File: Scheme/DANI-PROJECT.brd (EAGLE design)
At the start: 59.7 x 81 mm, 29 parts, among them T1 2N2222, T2 2N2222

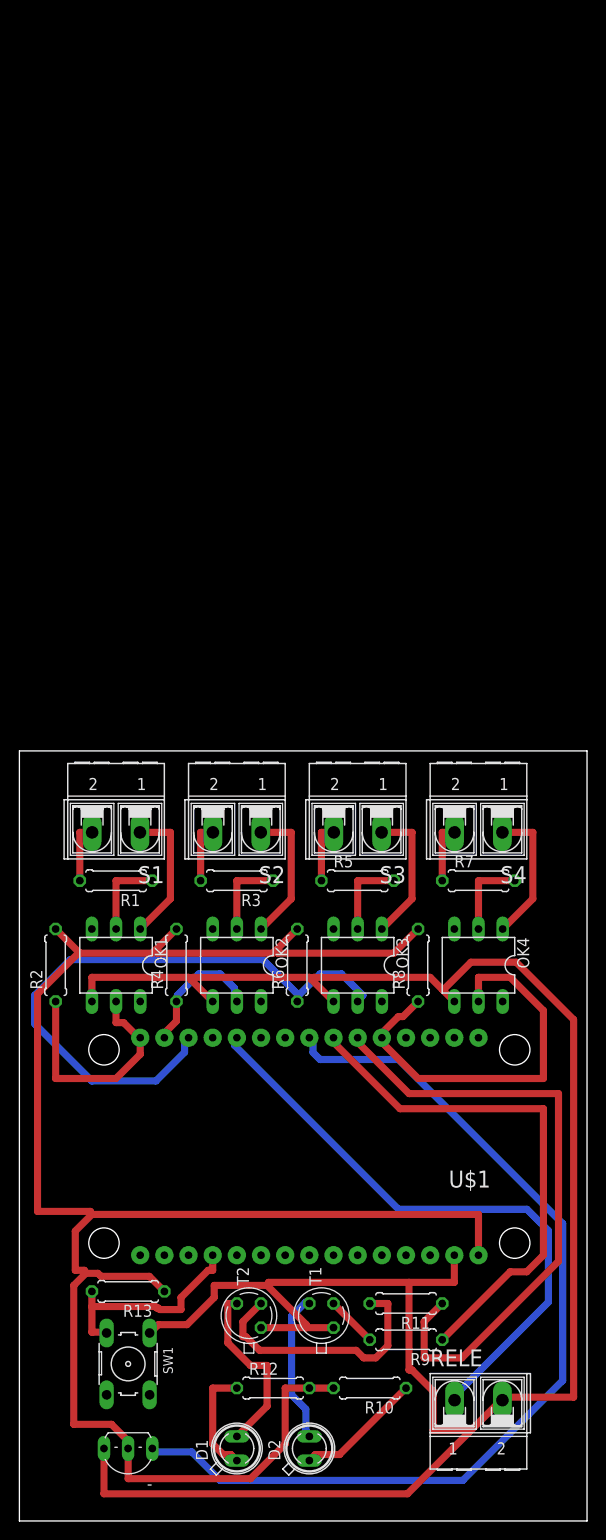
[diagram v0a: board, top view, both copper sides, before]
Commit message: simplified circuit
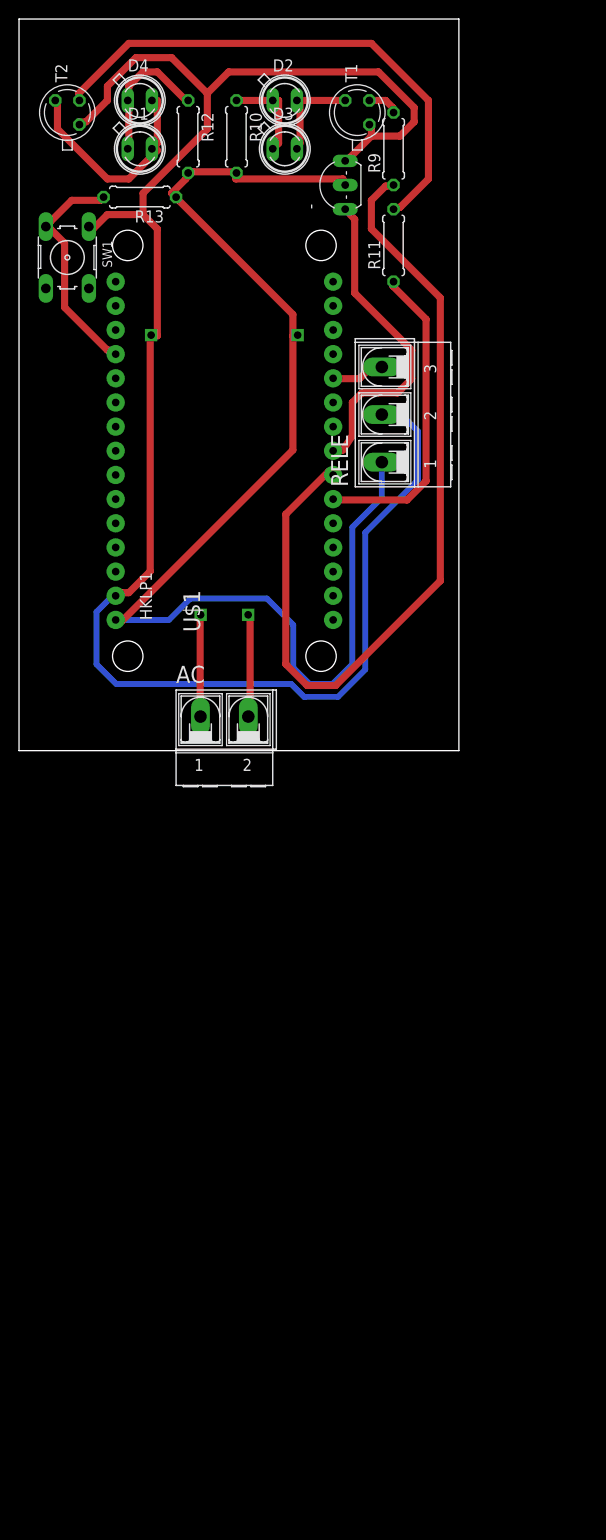
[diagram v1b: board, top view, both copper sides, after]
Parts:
- removed OK1, OK2, OK3, OK4: 4N25, optocoupler:DIL06
- removed R1, R3, R5, R7: 4k7, resistor:0207/7
- removed R2, R4, R6, R8: 10k, resistor:0207/7
- removed S1, S2, S3, S4: (no value), con-ptr500:AK500/2-H
- added AC: (no value), con-ptr500:AK500/2-H
- added D3, D4: SFH482, led:SFH482
- added HKLP1: HKLPM01, HKLPM01:HKLPM01
- RELE: device con-ptr500:AK500/2-H -> con-ptr500:AK500/3-H
- moved D2 141.7 mm to (27.9, 68.2), turned to 0 degrees
- moved D1 137.0 mm to (12.7, 63.2), turned to 0 degrees
- moved - 135.8 mm to (33.0, 59.4), turned to 90 degrees
- moved R10 132.3 mm to (22.8, 64.4), turned to 270 degrees
- moved R12 131.9 mm to (17.7, 64.4), turned to 270 degrees
- moved T2 127.9 mm to (5.04, 67.0)
- moved T1 126.5 mm to (35.5, 67.0)
- moved R9 125.2 mm to (39.3, 63.2), turned to 90 degrees
- moved SW1 116.5 mm to (5.04, 51.7)
- moved R13 115.0 mm to (12.7, 58.1)
- moved R11 111.2 mm to (39.3, 53.0), turned to 90 degrees
- moved RELE 104.1 mm to (38.1, 35.2), turned to 90 degrees
- moved U$1 73.7 mm to (21.6, 31.4), turned to 0 degrees
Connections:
- removed net N$10: R3.2, S2.2
- removed net N$11: R5.1, S3.2
- removed net N$12: OK3.1, S3.1
- removed net N$13: OK4.2, R7.2
- removed net N$14: OK4.1, S4.1
- removed net N$15: R7.1, S4.2
- removed net N$16: OK4.5, R8.1, U$1.D8
- removed net N$25: -.B, R10.2, R12.2, R13.1, R2.2, R4.2, R6.2, R8.2, U$1.VIN
- removed net N$3: OK1.1, S1.1
- removed net N$4: OK1.5, R2.1, U$1.D0
- removed net N$5: OK2.2, R3.1
- removed net N$6: OK3.2, R5.2
- removed net N$7: OK2.1, S2.1
- removed net N$8: OK2.5, R4.1, U$1.D1
- removed net N$9: OK3.5, R6.1, U$1.D2
- new net N$23: -.B, HKLP1.P$4, R10.2, R12.2, R13.1, RELE.1, U$1.VIN
- net N$1: now also AC.2, HKLP1.P$2; no longer OK1.2, R1.1
- net N$18: now also D4.K
- net N$2: now also AC.1, HKLP1.P$1; no longer R1.2, S1.2
- net N$21: now also D3.A
- net N$22: now also D3.K
- net N$24: now also D4.A
- net N$28: now also HKLP1.P$3; no longer OK1.4, OK2.4, OK3.4, OK4.4
- net N$31: now also RELE.3; no longer RELE.1
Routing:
- net N$25: track 199.7 -> 0.00 mm
- net N$23: track 0.00 -> 135.0 mm
- net N$29: track 101.0 -> 34.3 mm
- net N$9: track 65.4 -> 0.00 mm
- net N$31: track 63.9 -> 5.64 mm
- net N$28: track 236.4 -> 191.4 mm
- net N$16: track 42.8 -> 0.00 mm
- net N$26: track 55.2 -> 90.5 mm
- net N$27: track 66.3 -> 33.0 mm
- net N$19: track 27.3 -> 55.7 mm
- net N$4: track 25.2 -> 0.00 mm
- net N$14: track 14.7 -> 0.00 mm
- net N$3: track 14.7 -> 0.00 mm
- net N$7: track 14.7 -> 0.00 mm
- net N$12: track 14.7 -> 0.00 mm
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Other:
- board size 59.7 x 81 mm -> 46.2 x 76.9 mm
